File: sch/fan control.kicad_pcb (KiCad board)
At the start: 2 copper layers, 94 parts, among them J1 Serial Port, J2 Buttons, J3 Power 5V, J5 STATUS LEDs, J6 Light, J7 Motor cois, J8 AC 220v in, K1 SANYOU_SRD_Form_C, K2 SANYOU_SRD_Form_C, K3 SANYOU_SRD_Form_C, K4 SANYOU_SRD_Form_C, Q1 BC547, Q10 BT136-800, Q11 BC547, Q2 BC547, Q3 BC547, Q4 BC547, Q5 BC547, Q6 BC547, Q7 BC547, Q8 BC547, Q9 BC547, U1 PIC16F628-xxIP, U2 PC817, U3 PC817, U4 PC817, U5 PC817, U6 MOC3041M

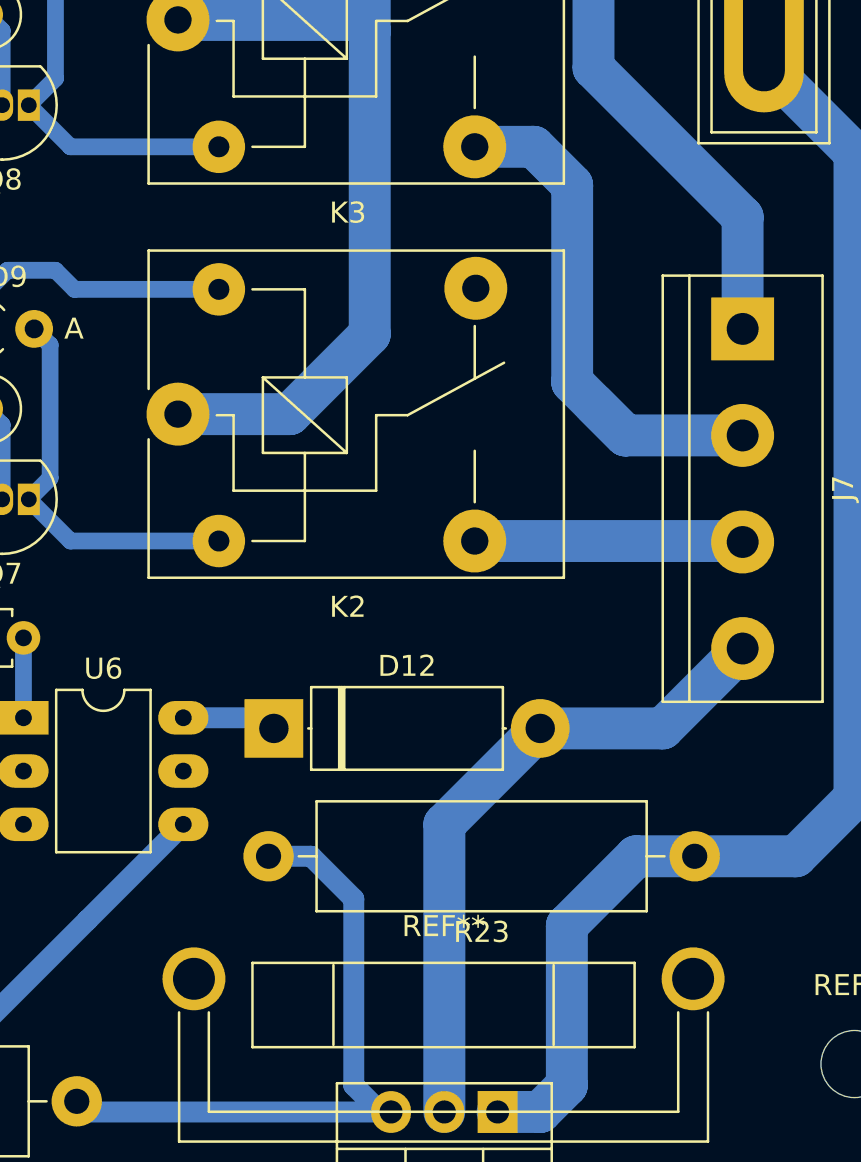
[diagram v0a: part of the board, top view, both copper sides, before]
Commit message: pcb
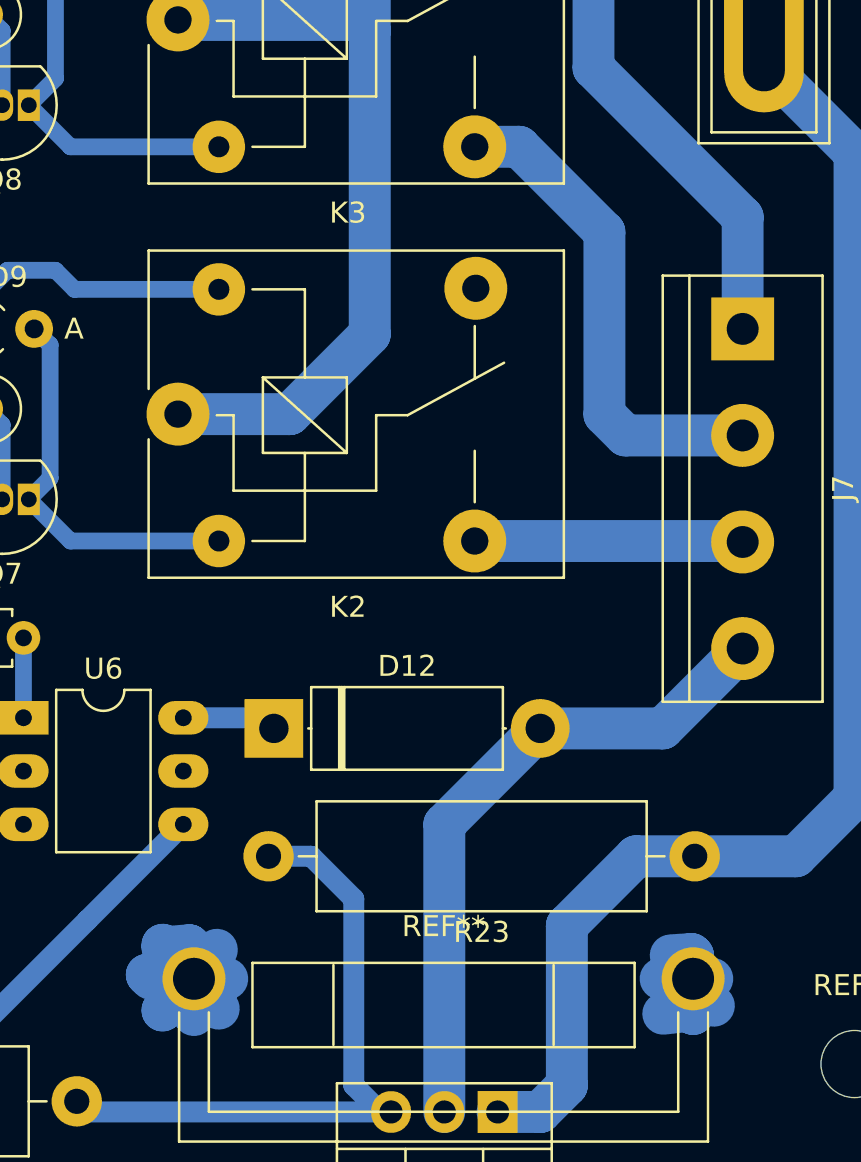
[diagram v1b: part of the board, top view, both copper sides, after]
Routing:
- net (no net): track 70.6 -> 95.0 mm
- net Net-(J7-Pad2): track 26.1 -> 23.6 mm
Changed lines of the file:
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@@
     (thickness 1.6)
     (drawings 1)
-    (tracks 487)
+    (tracks 513)
     (zones 0)
     (modules 94)
@@
   (segment (start 106.426 66.294) (end 115.824 66.294) (width 0.8) (layer F.Cu) (net 0))
   (segment (start 102.108 54.356) (end 96.266 54.356) (width 0.8) (layer F.Cu) (net 0))
+  (segment (start 160.02 112.7379) (end 160.02 113.03) (width 2) (layer B.Cu) (net 0))
+  (segment (start 161.1122 111.6457) (end 160.02 112.7379) (width 2) (layer B.Cu) (net 0))
+  (segment (start 160.02 113.2713) (end 161.2011 114.4524) (width 2) (layer B.Cu) (net 0))
+  (segment (start 160.02 113.2713) (end 160.02 113.03) (width 2) (layer B.Cu) (net 0))
+  (segment (start 158.520001 111.418499) (end 158.520001 111.530001) (width 2) (layer B.Cu) (net 0))
+  (segment (start 158.5341 111.4044) (end 158.520001 111.418499) (width 2) (layer B.Cu) (net 0))
+  (segment (start 160.02 113.03) (end 158.520001 114.529999) (width 2) (layer B.Cu) (net 0))
+  (segment (start 158.520001 114.542699) (end 158.520001 114.529999) (width 2) (layer B.Cu) (net 0))
+  (segment (start 160.02 114.7572) (end 160.02 113.03) (width 2) (layer B.Cu) (net 0))
+  (segment (start 160.02 111.6457) (end 159.8041 111.4298) (width 2) (layer B.Cu) (net 0))
+  (segment (start 160.02 113.03) (end 160.02 111.6457) (width 2) (layer B.Cu) (net 0))
+  (segment (start 158.520001 111.530001) (end 159.8041 111.4298) (width 2) (layer B.Cu) (net 0))
+  (segment (start 160.02 113.03) (end 161.6075 113.03) (width 2) (layer B.Cu) (net 0))
+  (segment (start 157.9626 113.03) (end 157.7721 112.8395) (width 2) (layer B.Cu) (net 0))
+  (segment (start 160.02 113.03) (end 157.7721 112.8395) (width 2) (layer B.Cu) (net 0))
+  (segment (start 183.82 113.03) (end 183.82 113.3223) (width 2) (layer B.Cu) (net 0))
+  (segment (start 183.82 113.3223) (end 184.8104 114.3127) (width 2) (layer B.Cu) (net 0))
+  (segment (start 183.82 113.0175) (end 183.82 113.03) (width 2) (layer B.Cu) (net 0))
+  (segment (start 183.82 113.03) (end 182.2704 113.03) (width 2) (layer B.Cu) (net 0))
+  (segment (start 183.82 111.9253) (end 183.7436 111.8489) (width 2) (layer B.Cu) (net 0))
+  (segment (start 183.82 113.03) (end 183.82 111.9253) (width 2) (layer B.Cu) (net 0))
+  (segment (start 183.7436 111.8489) (end 182.753 111.9124) (width 2) (layer B.Cu) (net 0))
+  (segment (start 183.82 113.03) (end 183.82 114.7062) (width 2) (layer B.Cu) (net 0))
+  (segment (start 183.82 114.7062) (end 183.6805 114.5667) (width 2) (layer B.Cu) (net 0))
+  (segment (start 183.6805 114.5667) (end 183.4896 114.5667) (width 2) (layer B.Cu) (net 0))
+  (segment (start 183.4896 114.5667) (end 182.3974 114.6937) (width 2) (layer B.Cu) (net 0))
+  (segment (start 184.7342 113.03) (end 183.82 113.03) (width 2) (layer B.Cu) (net 0))
   (segment (start 149.606 71.374) (end 145.796 75.184) (width 0.8) (layer B.Cu) (net 1))
   (segment (start 145.796 75.184) (end 143.256 75.184) (width 0.8) (layer B.Cu) (net 1))
@@
   (segment (start 173.408 92.156) (end 186.136 92.156) (width 2) (layer B.Cu) (net 30))
   (segment (start 180.594 87.122) (end 186.182 87.122) (width 2) (layer B.Cu) (net 31))
-  (segment (start 179.07 85.598) (end 180.594 87.122) (width 2) (layer B.Cu) (net 31))
-  (segment (start 173.408 73.36) (end 176.23 73.36) (width 2) (layer B.Cu) (net 31))
-  (segment (start 176.23 73.36) (end 178.054 75.184) (width 2) (layer B.Cu) (net 31))
-  (segment (start 178.054 84.582) (end 180.594 87.122) (width 2) (layer B.Cu) (net 31))
-  (segment (start 178.054 75.184) (end 178.054 84.582) (width 2) (layer B.Cu) (net 31))
+  (segment (start 179.5907 86.1187) (end 180.594 87.122) (width 2) (layer B.Cu) (net 31))
+  (segment (start 179.5907 77.42138) (end 179.5907 86.1187) (width 2) (layer B.Cu) (net 31))
+  (segment (start 175.52932 73.36) (end 179.5907 77.42138) (width 2) (layer B.Cu) (net 31))
+  (segment (start 173.408 73.36) (end 175.52932 73.36) (width 2) (layer B.Cu) (net 31))
   (segment (start 173.408 54.564) (end 176.738 54.564) (width 2) (layer B.Cu) (net 32))
   (segment (start 176.738 54.564) (end 179.07 56.896) (width 2) (layer B.Cu) (net 32))
